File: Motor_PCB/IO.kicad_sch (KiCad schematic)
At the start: 54 parts, among them Q401 BC846, Q402 TPH4R50ANH1, Q403 TPH4R50ANH1, Q404 2N7002, Q405 2N7002, Q406 BC856, U401 VOM1271T, U402 TCAN1043H

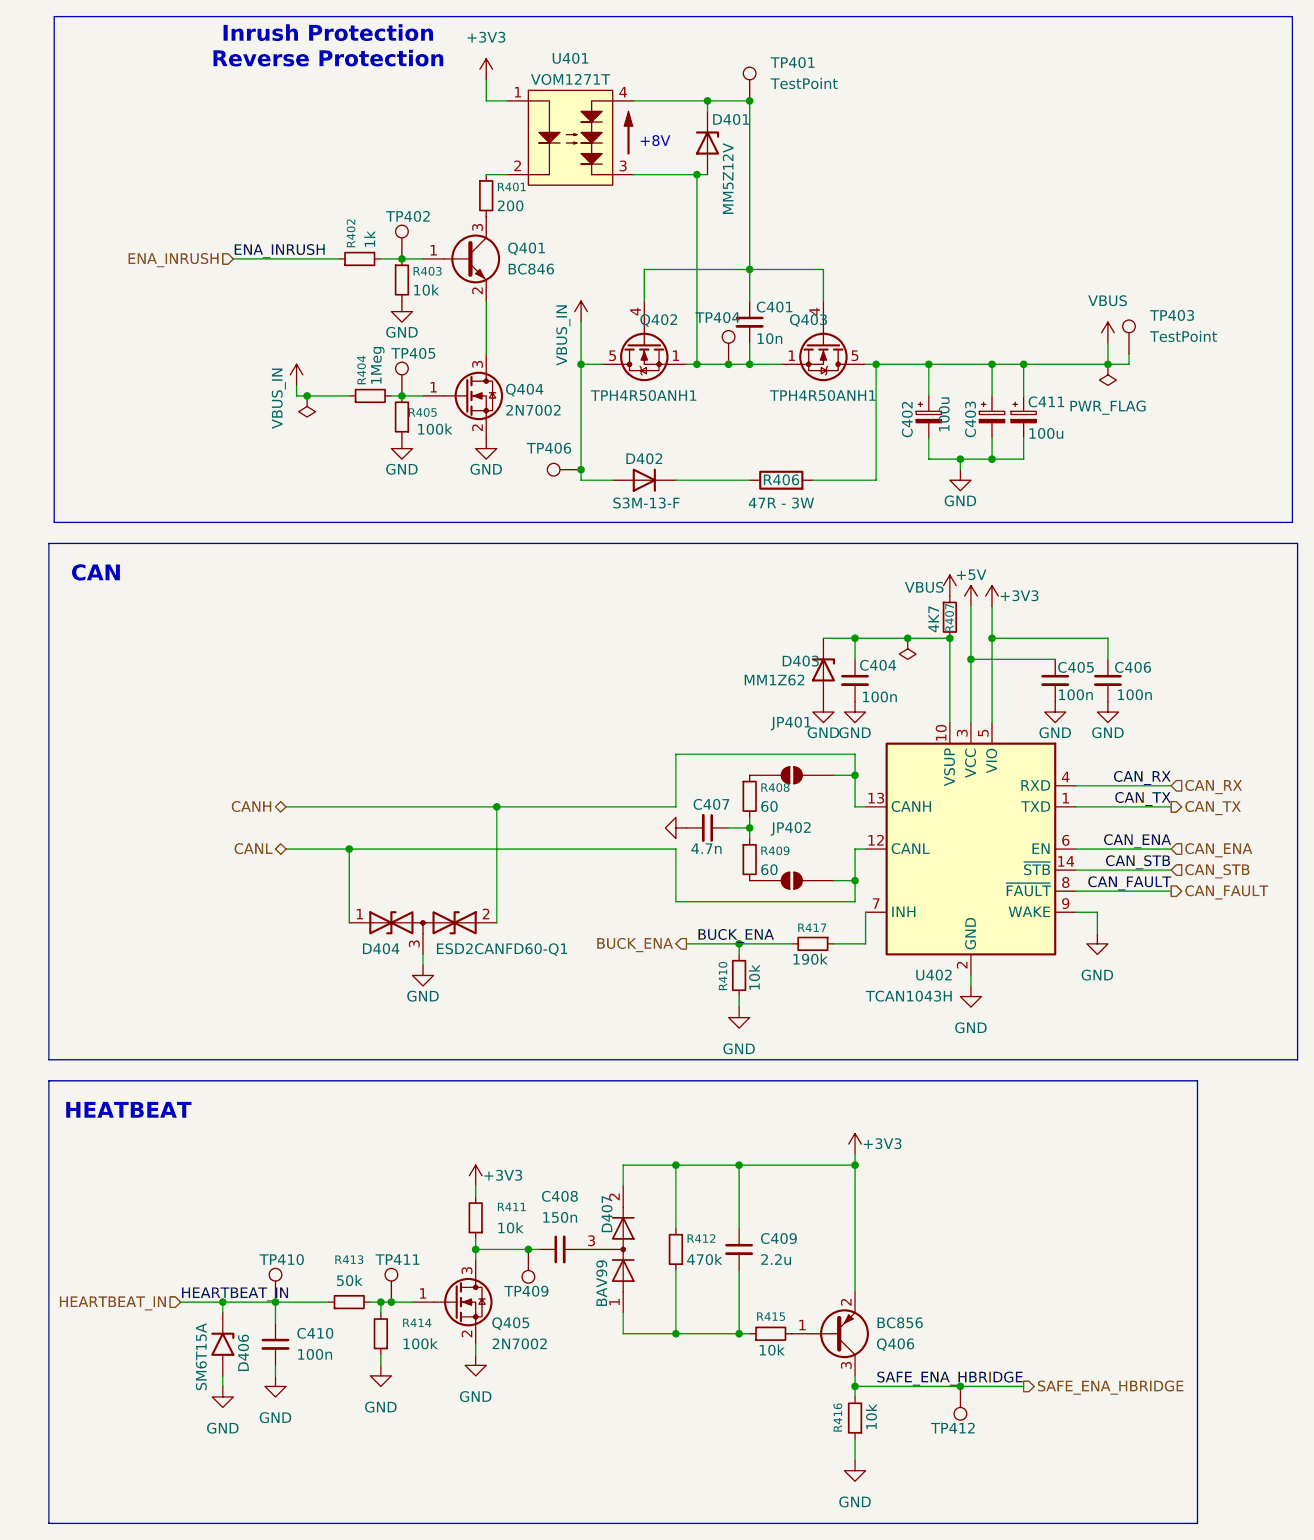
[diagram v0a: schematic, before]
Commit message: 20/10-2026
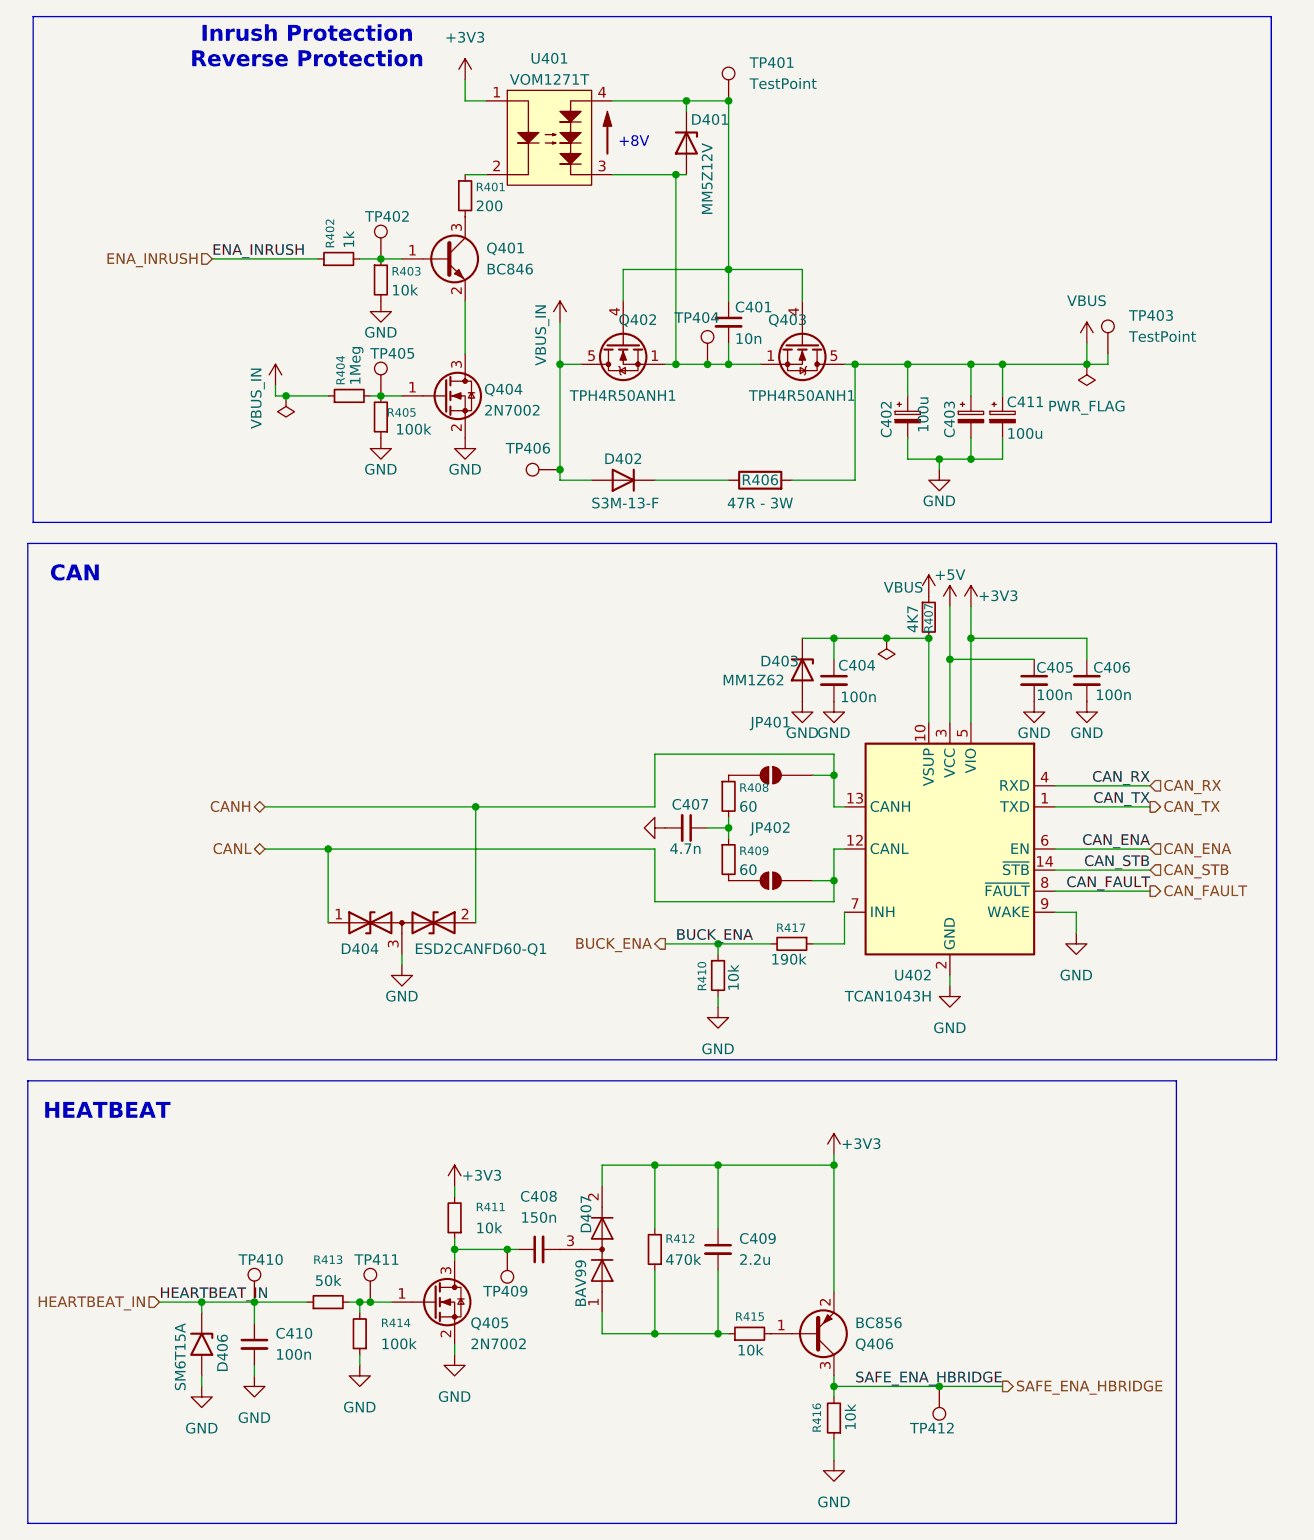
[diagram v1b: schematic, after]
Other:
- moved on the sheet: C401, C402, C403, C404, C405, C406, C407, C408, C409, C410, C411, D401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
